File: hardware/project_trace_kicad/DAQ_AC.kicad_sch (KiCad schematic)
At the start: 55 parts, among them U301 THS4131IDR, U303 ADS1602, U304 MCP6499T, U306 LM4040DBZ-4.1

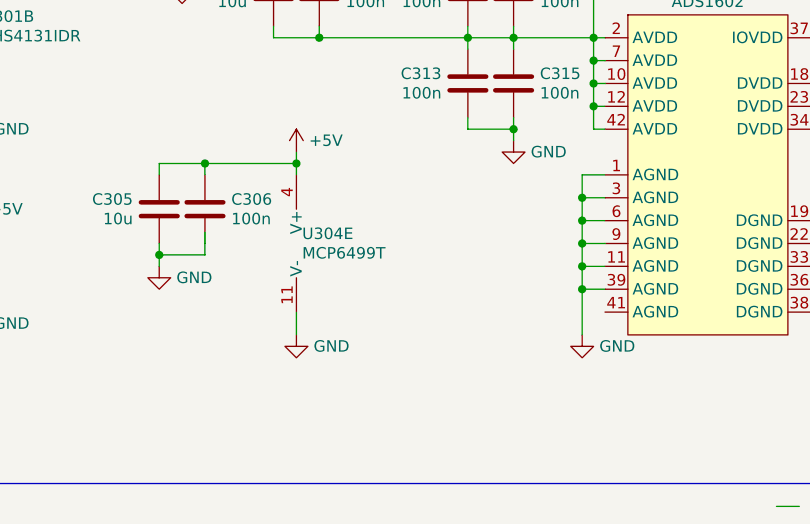
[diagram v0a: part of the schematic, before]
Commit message: Before using stashed changes
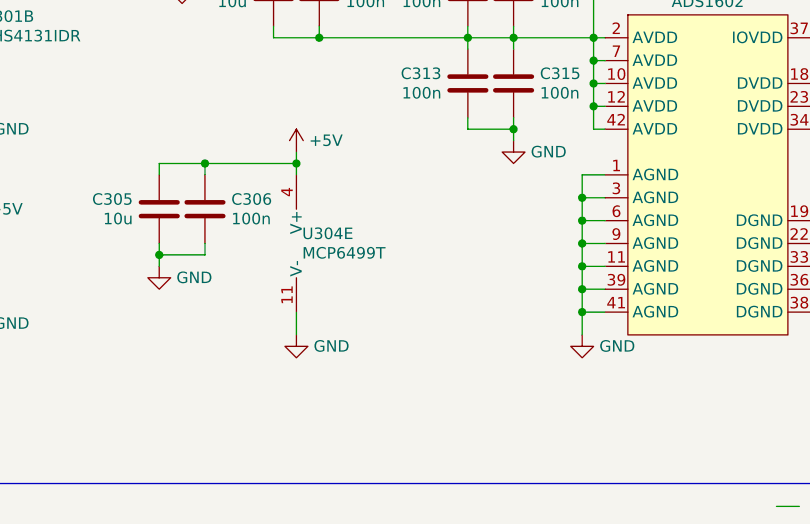
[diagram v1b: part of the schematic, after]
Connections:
- net GND: now also U303.41 (AGND)
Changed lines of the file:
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@@
+	)
+	(junction
+		(at 118.11 143.51)
+		(diameter 0)
+		(color 0 0 0 0)
 	)
 	(junction
@@
 	(wire
 		(pts
-			(xy 76.2 134.62) (xy 76.2 135.89)
+			(xy 118.11 143.51) (xy 120.65 143.51)
 		)
 		(stroke
@@
 	(wire
 		(pts
-			(xy 118.11 140.97) (xy 118.11 146.05)
+			(xy 118.11 140.97) (xy 118.11 143.51)
 		)
 		(stroke
@@
 		)
 		(stroke
+			(width 0)
+			(type default)
+		)
+	)
+	(wire
+		(pts
+			(xy 118.11 143.51) (xy 118.11 146.05)
+		)
+		(stroke
